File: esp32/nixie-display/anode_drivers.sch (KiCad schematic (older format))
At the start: 49 parts, among them J2 Conn_02x10_Odd_Even, Q1 MPSA42, Q10 MPSA92, Q11 MPSA42, Q12 MPSA92, Q13 MPSA42, Q14 MPSA92, Q2 MPSA92, Q3 MPSA42, Q4 MPSA92, Q5 MPSA42, Q6 MPSA92, Q7 MPSA42, Q8 MPSA92, Q9 MPSA42

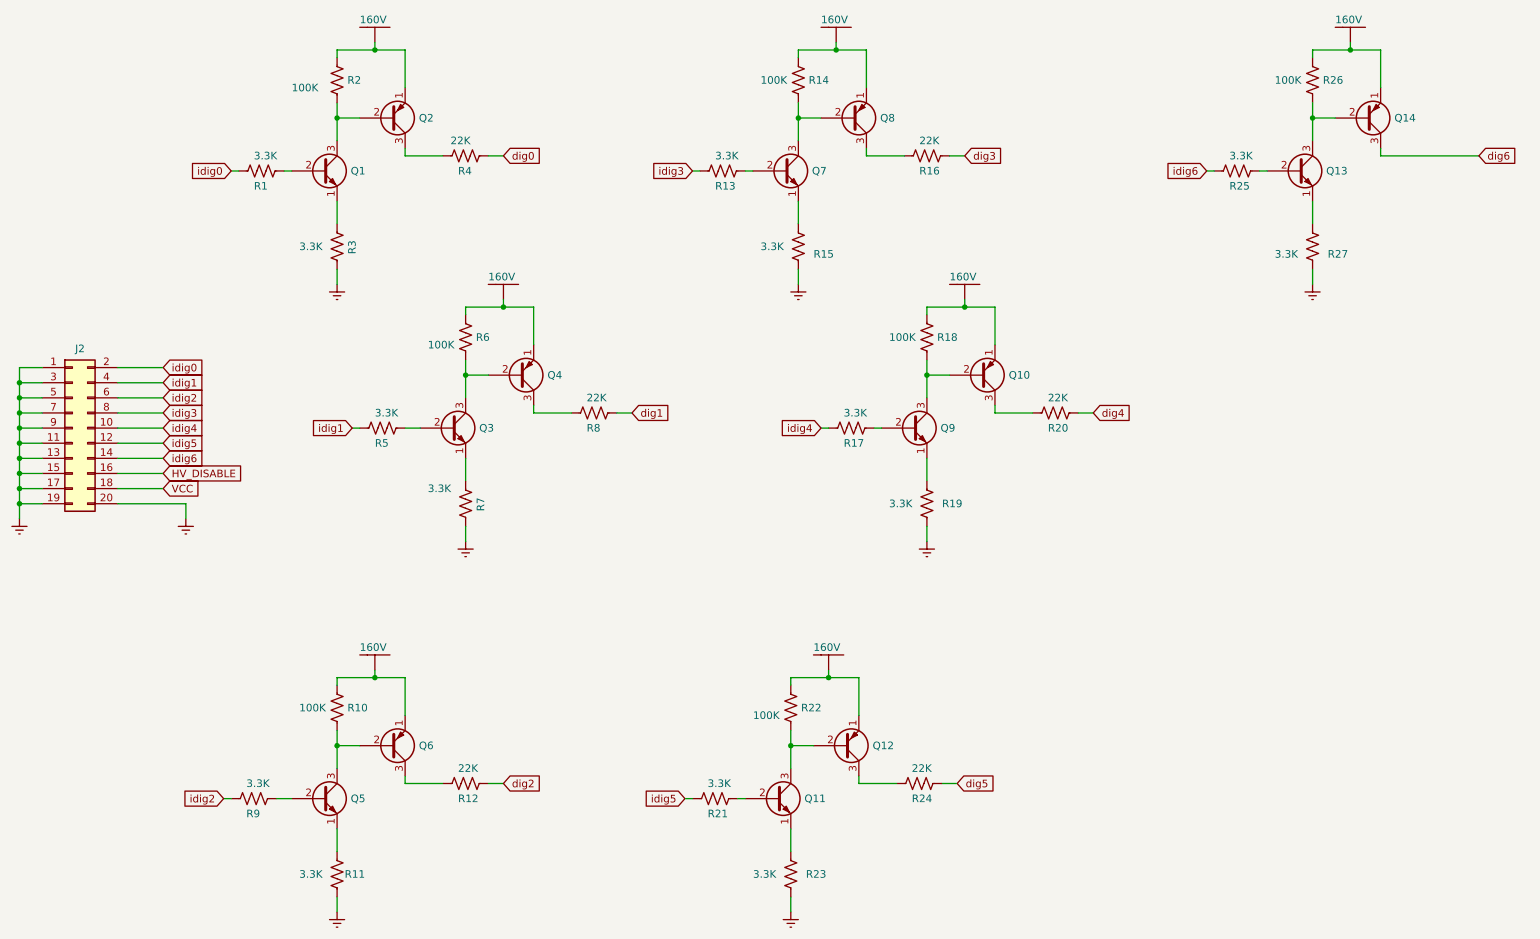
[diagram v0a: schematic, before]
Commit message: New Zen design
[git-p4: depot-paths = "//depot/nixiestat/": change = 356]
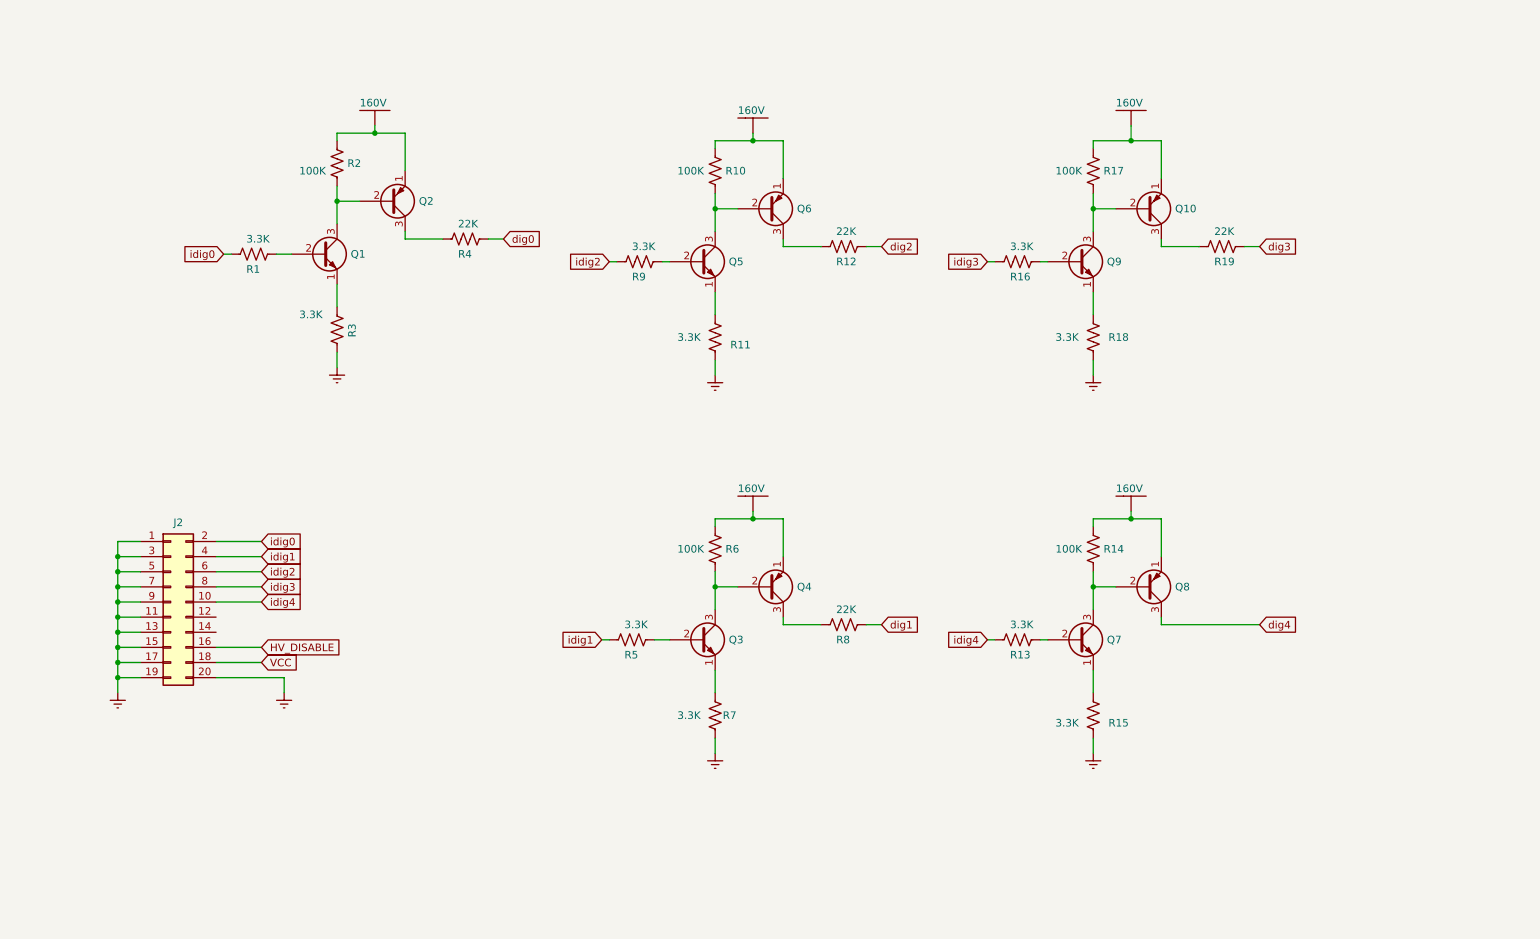
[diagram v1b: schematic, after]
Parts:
- removed Q1, Q11: MPSA42, Package_TO_SOT_THT:TO-92L_Inline_Wide, symbol Device:Q_NPN_EBC
- removed Q12, Q2: MPSA92, Package_TO_SOT_THT:TO-92L_Inline_Wide, symbol Device:Q_PNP_EBC
- removed R1, R21, R23, R3: 3.3K, Resistor_SMD:R_0805_2012Metric_Pad1.20x1.40mm_HandSolder, symbol Device:R_US
- removed R2, R22: 100K, Resistor_SMD:R_0805_2012Metric_Pad1.20x1.40mm_HandSolder, symbol Device:R_US
- removed R24, R4: 22K, Resistor_SMD:R_1206_3216Metric_Pad1.30x1.75mm_HandSolder, symbol Device:R_US
- removed V2, V7: 160V, symbol croftj:160V
- renumbered Q3 to Q1, Q4 to Q2, Q5 to Q3, Q6 to Q4, Q7 to Q5, Q8 to Q6, Q13 to Q7, Q14 to Q8, R5 to R1, R14 to R10, R15 to R11, R16 to R12, R25 to R13, R26 to R14, R27 to R15, R17 to R16, R18 to R17, R19 to R18, R20 to R19, R6 to R2, R7 to R3, R8 to R4, R9 to R5, R10 to R6, R11 to R7, R12 to R8, R13 to R9
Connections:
- net dig6 is gone; now on net dig4: Q8.3 (C)
- net dig0: now also R4.1
- net dig1: now also R8.1; no longer R4.1
- net dig2: now also R12.1; no longer R8.1
- net dig3: now also R19.1; no longer R12.1
- net dig4: no longer R19.1
- net idig0: now also R1.2
- net idig1: now also R5.2; no longer R1.2
- net idig2: now also R9.2; no longer R5.2
- net idig3: now also R16.2; no longer R9.2
- net idig4: now also R13.2; no longer R16.2
- net idig5: no longer names the net of J2.12 (Pin_12)
- net idig6: no longer names the net of J2.14 (Pin_14)
- net idig6: no longer R13.2
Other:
- moved on the sheet: J2, Q1, Q10, Q2, Q3, Q4, Q5, Q6, Q7, Q8, Q9, R1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
